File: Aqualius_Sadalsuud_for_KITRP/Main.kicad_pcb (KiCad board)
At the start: 2 copper layers, 100 x 100 mm, 341 parts, among them J1 microSD, J10 I/O_Vdd, J11 ENC1, J12 ENC0, J13 ENC3, J14 ENC2, J15 5Vin, J16 EMG, J17 MOTOR0, J18 MOTOR1, J19 MOTOR2, J2 ADC, J20 MOTOR3, J21 MOTOR4, J22 MOTOR5, J23 BATT_IN, J24 BATT_IN, J25 FUSE, J27 Advanced_SBDBT, J28 PICkit3, J3 SWD, J4 CAN, J5 ADC_Vdd, J6 SERIAL0, J7 CAN, J8 VALVE, J9 SERIAL2, Q1 NPN, Q10 NVMFD5C446NLT1G, Q11 FET_N, Q12 NVMFD5C446NLT1G, Q13 NVMFD5C446NLT1G, Q14 NVMFD5C446NLT1G, Q15 NVMFD5C446NLT1G, Q16 NVMFD5C446NLT1G, Q17 NVMFD5C446NLT1G, Q18 FET_P, Q2 FET_P, Q3 FET_P, Q4 FET_P, Q5 NVMFD5C446NLT1G, Q6 NVMFD5C446NLT1G, Q7 NVMFD5C446NLT1G, Q8 NVMFD5C446NLT1G, Q9 NVMFD5C446NLT1G, SW1 RESET, SW10 TOGGLESW1, SW11 TOGGLESW2, SW12 TOGGLESW3, SW2 TOGGLESW0, SW3 SW0, SW4 SW1, SW5 Control-Power_SW, SW6 SW2, SW7 SW3, SW8 EMG_SW, SW9 MAIN_SW, U1 MAX3051, U10 BD9G101G, U11 CCG30-24-12, U12 NCP5104, U13 NCP5104, U14 NCP5104, U15 NCP5104, U16 NCP5104, U17 NCP5104, U18 V23086-C1001, U19 NCP5104, U2 BD9G101G, U20 NCP5104, U21 NCP5104, U22 NCP5104, U23 NCP5104, U24 NCP5104, U25 LOGO, U26 7805, U27 TBD62083A, U28 LOGO, U29 LOGO, U30 LM7812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

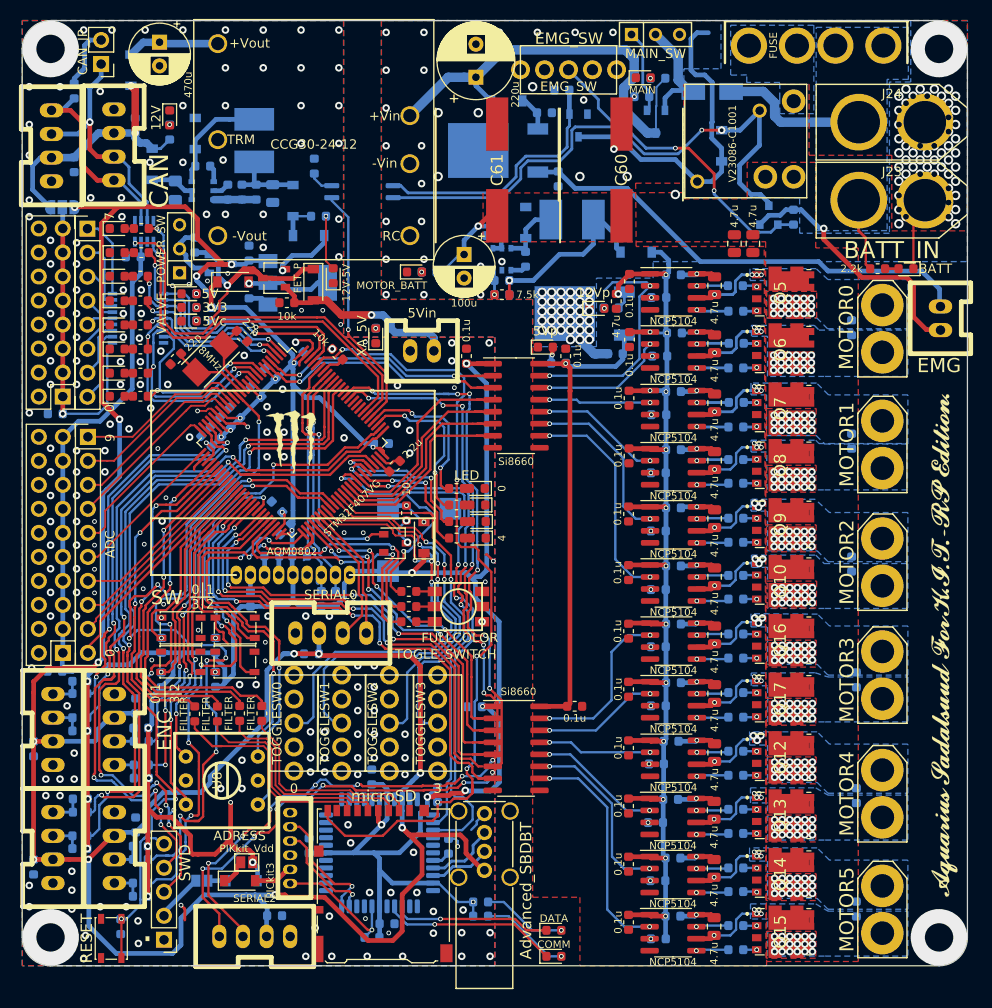
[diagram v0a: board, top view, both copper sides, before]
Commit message: for KIT-RP
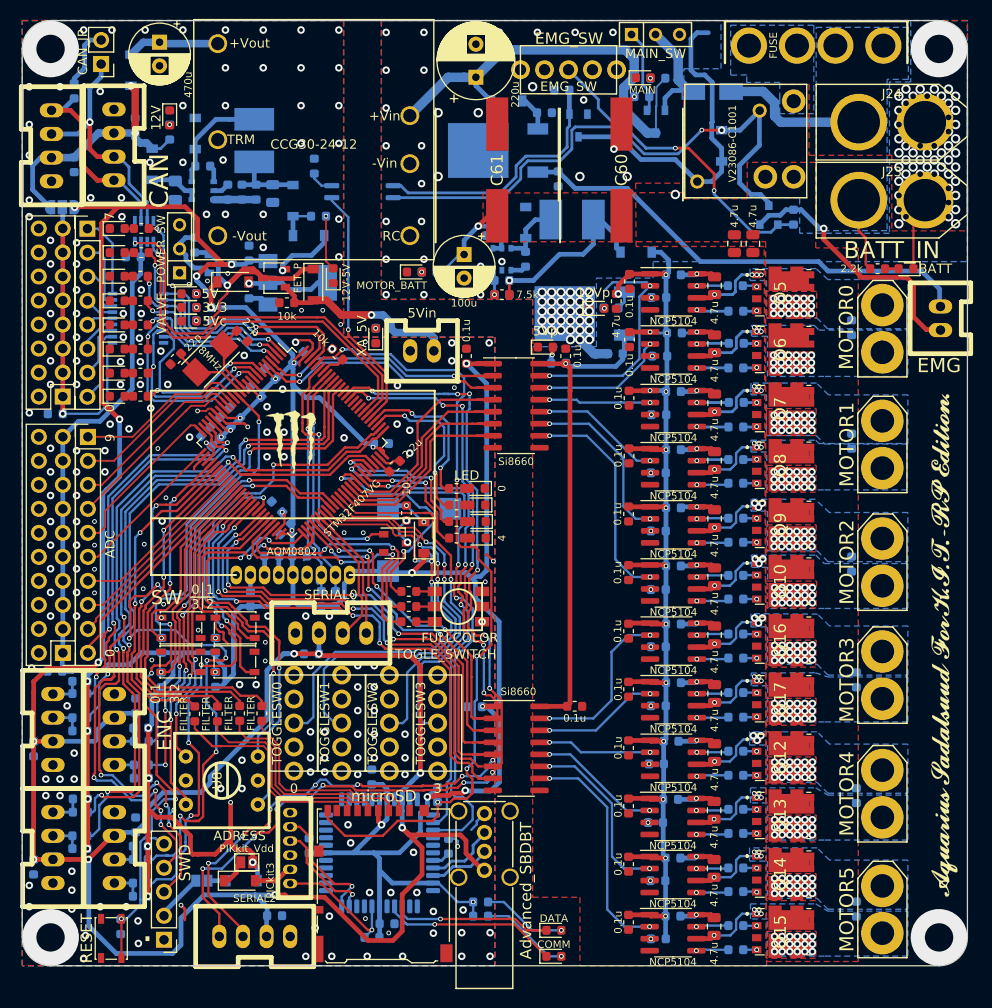
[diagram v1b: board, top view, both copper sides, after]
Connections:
- net /~RST renamed /~{RST}
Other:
- net class Default removed
